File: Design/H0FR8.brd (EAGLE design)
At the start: 34.6 x 30 mm, 24 parts, among them P1 HEXABIT_17.32_NO_P6, Q1 TLP184_GR-TPL,SE, U1 STM32G0B1CEU6N, U2 T2035H-6GD2PAK_T2550_STM-M, U3 VOT8121AM-VT, X1 XTALL_CSTCE8M00G52

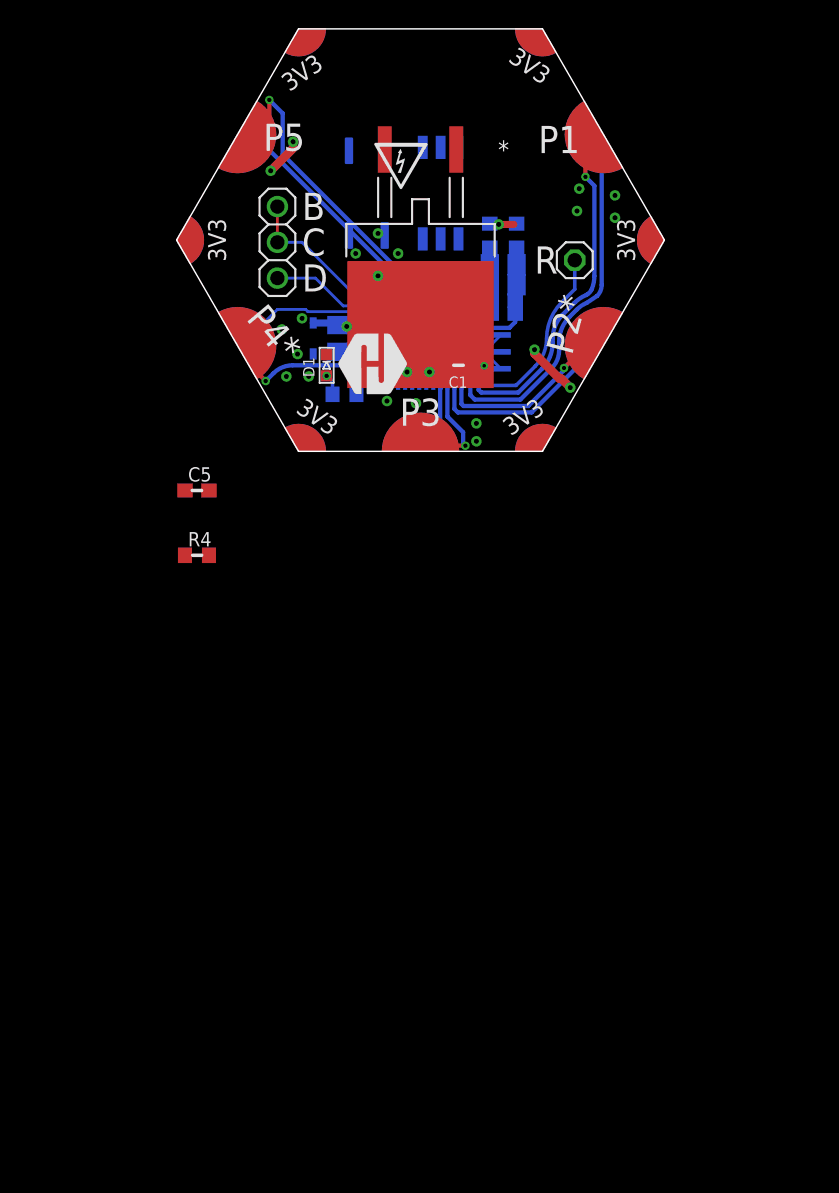
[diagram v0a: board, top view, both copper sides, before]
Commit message: Stage1
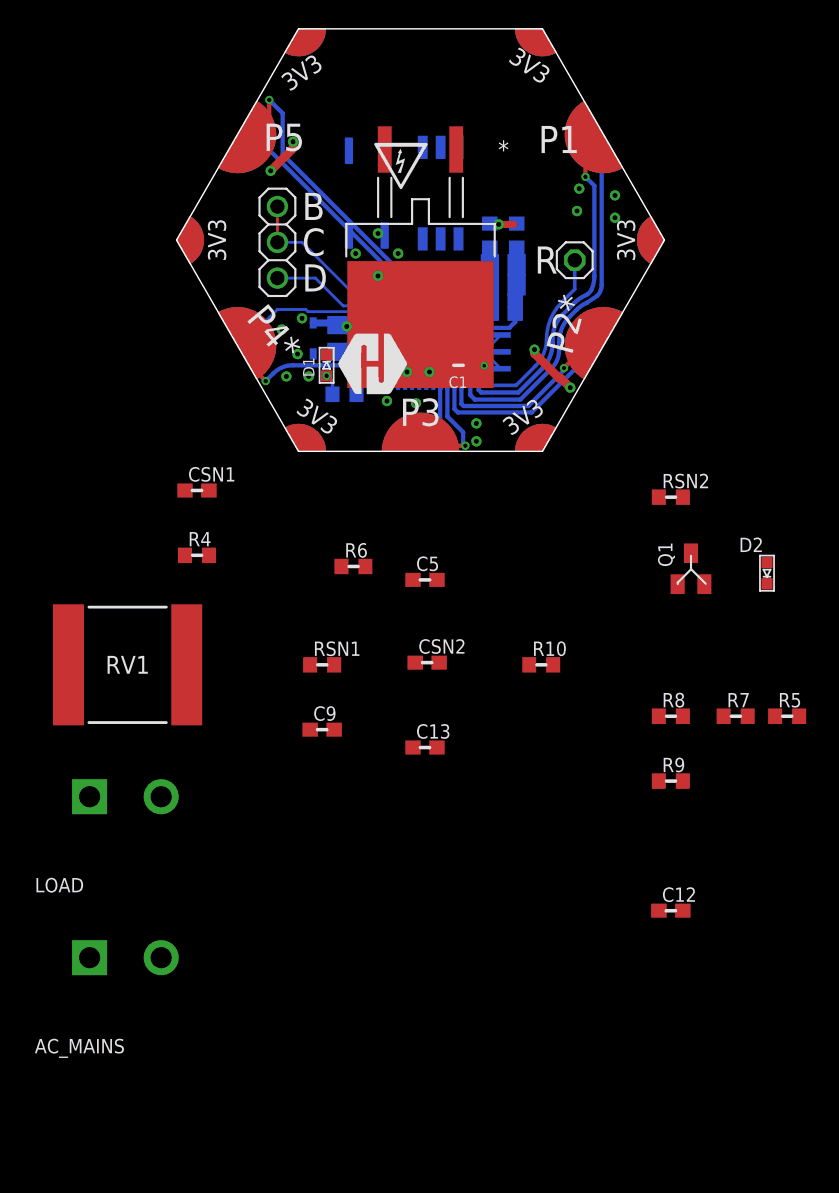
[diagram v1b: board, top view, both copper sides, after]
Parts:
- added AC_MAINS, LOAD: (no value), HEXABITZ_CONNECTION_PARTS:1546111-2
- added C12, CSN2: 100nF, HEXABITZ_RCLS:C-0603
- added C13: 1nF, HEXABITZ_RCLS:C-0603
- added C9, CSN1: 10nF, HEXABITZ_RCLS:C-0603
- added D2: RED, Hexabitz:VLMS1300-GS08
- added R10, R5, RSN1: 100, HEXABITZ_RCLS:R-0603
- added R6: 390, HEXABITZ_RCLS:R-0603
- added R7: 180, HEXABITZ_RCLS:R-0603
- added R8: 3.3k, HEXABITZ_RCLS:R-0603
- added R9: 47, HEXABITZ_RCLS:R-0603
- added RSN2: 1.5k, HEXABITZ_RCLS:R-0603
- added RV1: MOVS4032V275, HEXABITZ_RCLS:MOVS4032V275
- added U4: TLP184_GR-TPL,SE, HEXABITZ_ICs:SOIC127P700X230-6N
- C5: value 100nF -> 1nF
- Q1: value TLP184_GR-TPL,SE -> MMBT3904LT1; device HEXABITZ_ICs:SOIC127P700X230-6N -> HEXABITZ_RCLS:MMBT3904LT1
- R4: value 0.0R -> 1k
- moved Q1 32.1 mm to (19.2, -8.41), flipped to the top, turned to 0 degrees
- moved C5 17.4 mm to (0.32, -9.21)
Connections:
- new net A2: LOAD.2, RSN1.2, RSN2.2, RV1.1, U2.2
- new net AC_MAINS_L: AC_MAINS.1, LOAD.1
- new net AC_MAINS_N: AC_MAINS.2, C9.2, CSN1.2, CSN2.2, R4.1, RV1.2, U2.1
- new net N$10: C12.1, R5.2, R9.2
- new net N$11: C12.2, Q1.3, R5.1
- new net N$12: R9.1, U3.2
- new net N$13: C5.1, Q1.1, R8.1
- new net N$4: CSN1.1, RSN1.1
- new net N$7: CSN2.1, R6.2, RSN2.1
- new net N$8: R6.1, U3.4
- new net N$9: D2.C, R7.2
- new net TRIAC_G: C9.1, R4.2, U2.3, U3.3
- new net ZC_DETECT: C13.1, R10.2, U4.6
- net GND: now also C13.2, Q1.2, U4.4
- net SSR: now also C5.2, R8.2
- net VDD: now also D2.A, R10.1, U3.1

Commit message: stage2
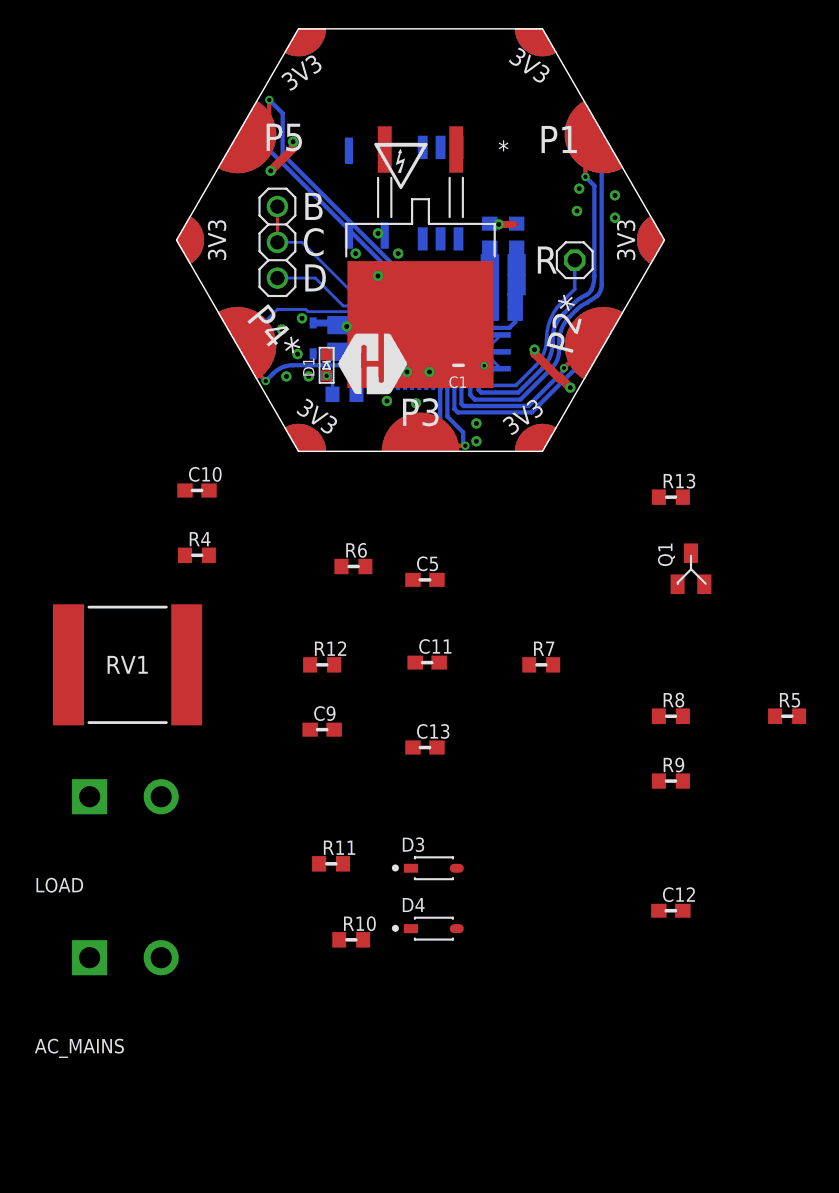
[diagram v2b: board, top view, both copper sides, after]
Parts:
- added D4: STMICROELECTRONICS_BAT46ZFILMSTMICROELECTRONICS_BAT46ZFILM_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, HEXABITZ_RCLS:STMICROELECTRONICS_BAT46ZFILM_3
- added R11: 100k, HEXABITZ_RCLS:R-0603
- D2: value RED -> BOURNS_CDSOD323-T03SCBOURNS_CDSOD323-T03SC_0_0; device Hexabitz:VLMS1300-GS08 -> HEXABITZ_RCLS:BOURNS_CDSOD323-T03SC_0
- D3: value BOURNS_CDSOD323-T03SCBOURNS_CDSOD323-T03SC_0_0 -> STMICROELECTRONICS_BAT46ZFILMSTMICROELECTRONICS_BAT46ZFILM_0_3; device HEXABITZ_RCLS:BOURNS_CDSOD323-T03SC_0 -> HEXABITZ_RCLS:STMICROELECTRONICS_BAT46ZFILM_3
- R10: value 100 -> 100k
- R7: value 180 -> 33k
- moved D3 38.6 mm to (0.95, -29.7), flipped to the top, turned to 0 degrees
- moved D2 36.3 mm to (-7.62, 7.94), flipped to the bottom, turned to 270 degrees
- moved R10 23.7 mm to (-4.92, -34.8)
- moved R7 14.3 mm to (8.57, -15.2)
- renumbered CSN1 to C10, CSN2 to C11, RSN1 to R12, RSN2 to R13
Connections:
- removed net N$9: D2.C, R7.2
- new net N$14: D3.2, D4.2
- new net N$15: D3.1, R11.1, U4.1
- new net N$16: D4.1, R10.1, U4.3
- net AC_MAINS_L: now also R11.2
- net AC_MAINS_N: now also R10.2
- net GND: now also D2.2; no longer D3.2
- net VDD: now also D2.1, R7.1; no longer D2.A, D3.1, R10.1
- net ZC_DETECT: now also R7.2; no longer R10.2

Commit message: Final schematic design
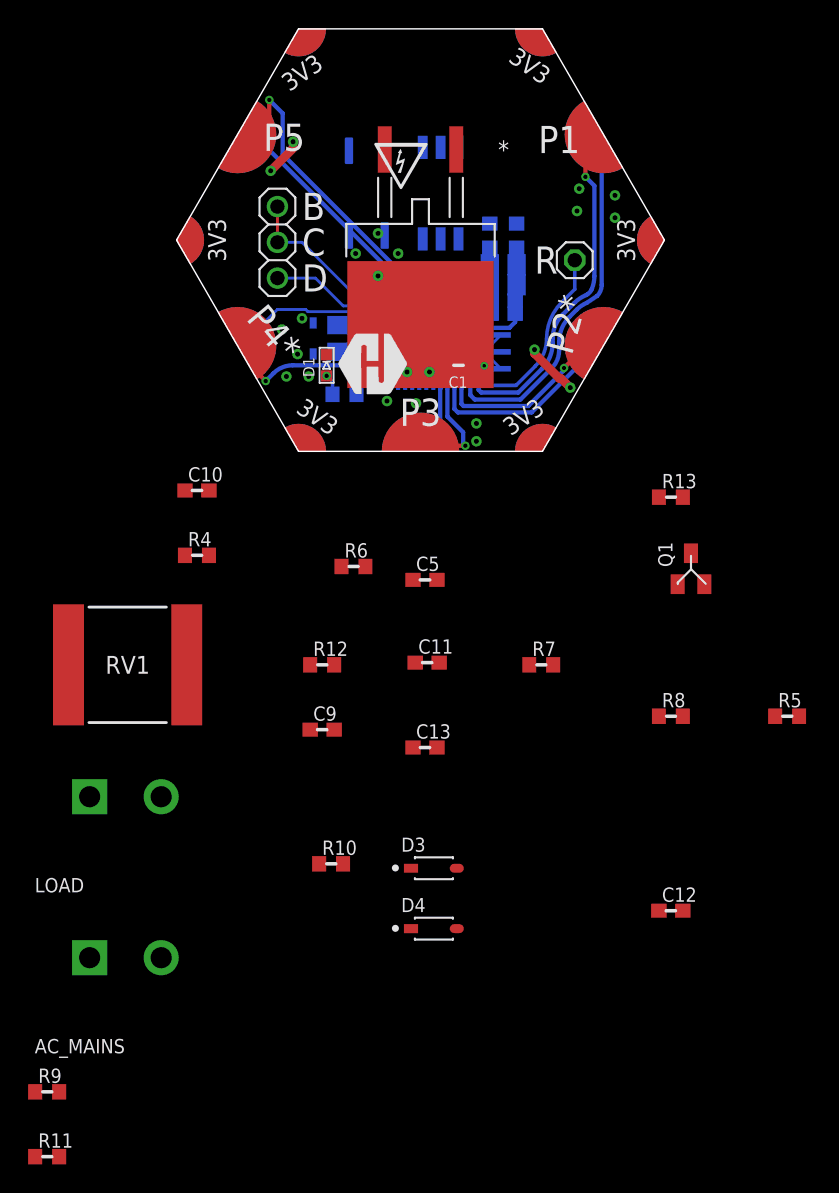
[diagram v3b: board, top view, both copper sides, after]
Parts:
- C11: value 100nF -> 47nF
- moved R9 49.5 mm to (-26.5, -45.6)
- moved R11 29.0 mm to (-26.5, -50.2)
- moved R10 5.58 mm to (-6.35, -29.4)
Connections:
- net N$3 renamed LED_INDICATOR
- removed net N$12: R9.1, U3.2
- removed net SSR: C5.2, R8.2, U1.43
- new net AGND: C3.2, C7.2, R3.2, U1.7
- new net N$3: R9.1, U3.1
- new net TRIAC_TRIGGER: C5.2, R8.2, U1.20
- net AC_MAINS_L: now also R10.2; no longer R11.2
- net AC_MAINS_N: now also R11.2; no longer R10.2
- net GND: now also R3.1; no longer R3.2
- net N$10: now also U3.2; no longer R9.2
- net N$15: now also R10.1; no longer R11.1
- net N$16: now also R11.1; no longer R10.1
- net VDD: now also FB1.1, R9.2; no longer FB1.2, U3.1
- net VDDA: now also FB1.2; no longer FB1.1
- net VSSA: no longer C3.2, C7.2, R3.1, U1.7
- net ZC_DETECT: now also U1.19
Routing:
- net VDD: track 6.79 -> 0.94 mm, vias 2 -> 0
- net LED_INDICATOR: track 2.14 -> 0.00 mm
- net SSR: track 1.23 -> 0.00 mm
- net VSSA: track 4.72 -> 3.74 mm
- net GND: track 10.8 -> 9.81 mm
